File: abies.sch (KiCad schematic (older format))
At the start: 33 parts

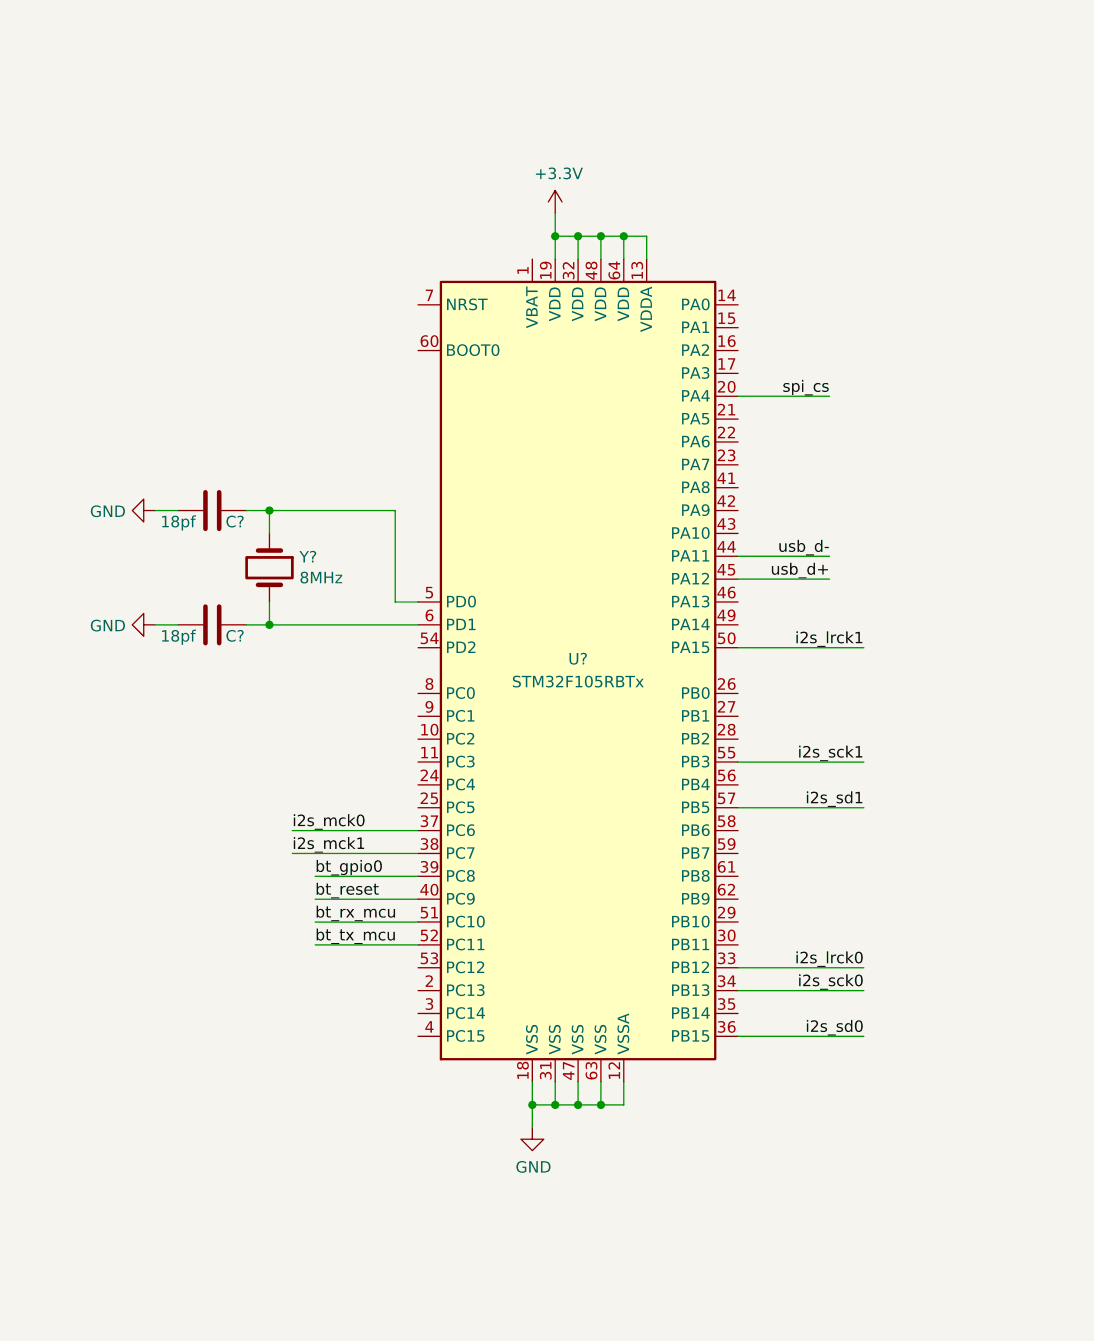
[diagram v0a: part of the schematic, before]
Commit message: Fix stuff. add psoc to sch
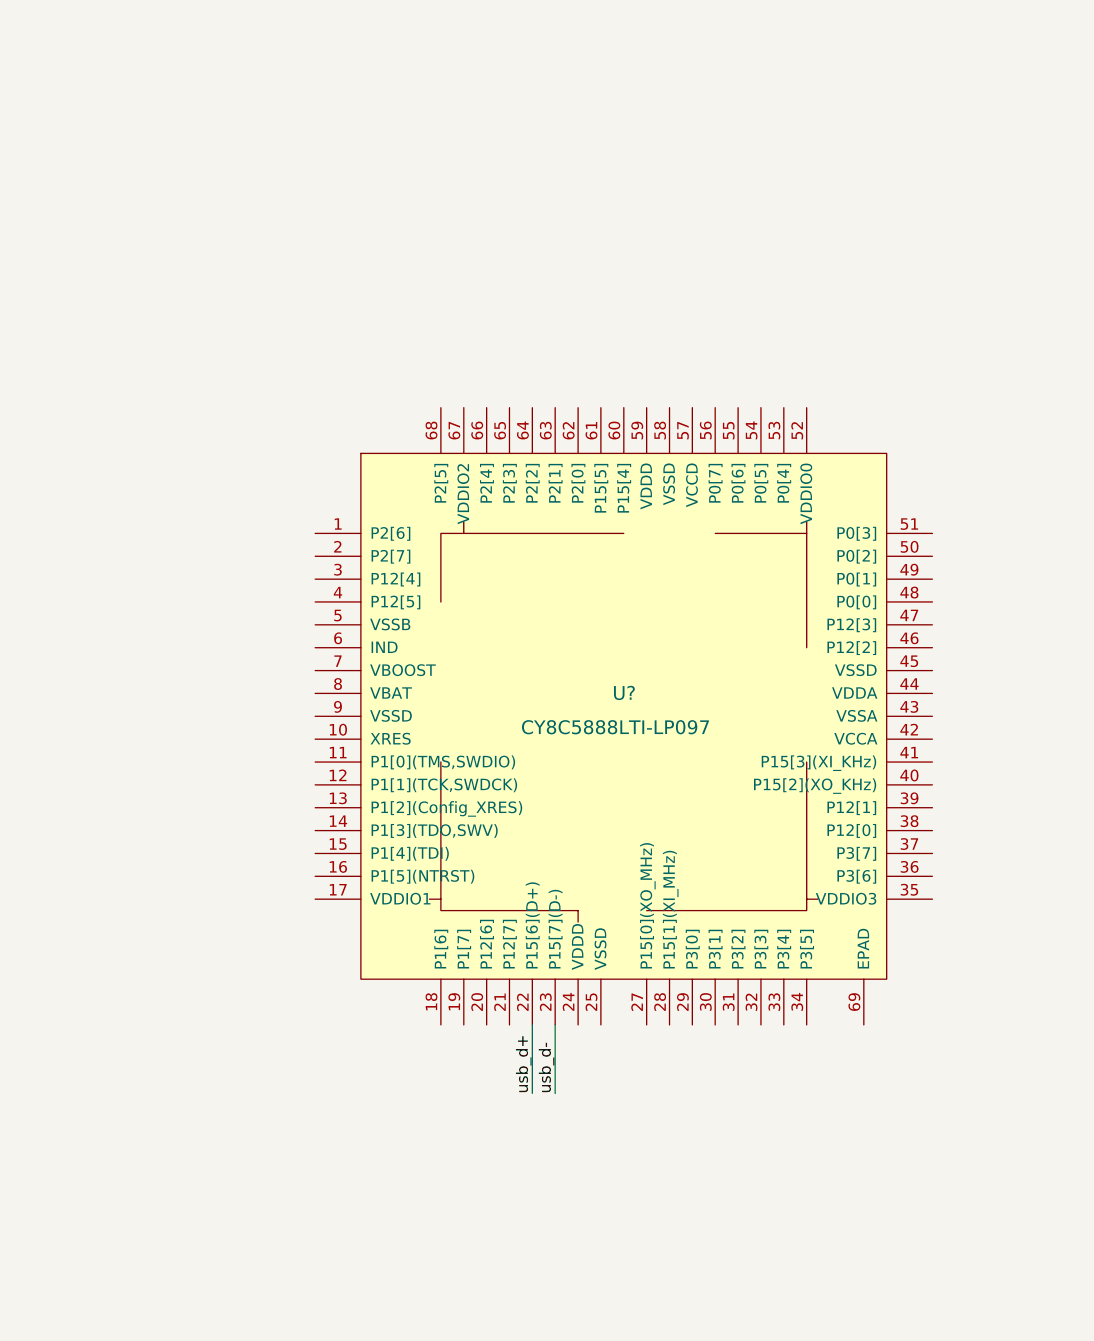
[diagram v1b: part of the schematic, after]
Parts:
- removed C? (x2): 18pf, symbol Device:C
- removed U?: STM32F105RBTx, Package_QFP:LQFP-64_10x10mm_P0.5mm, symbol MCU_ST_STM32F1:STM32F105RBTx
- removed Y?: 8MHz, symbol Device:Crystal
- added U?: CY8C5888LTI-LP097, Package_DFN_QFN:QFN-68-1EP_8x8mm_P0.4mm_EP5.2x5.2mm_ThermalVias, symbol microcontroller_arm:CY8C5888LTI-LP097
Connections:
- net usb_d+: now also U?.22 (P15[6](D+))
- net usb_d-: now also U?.23 (P15[7](D-))
- new net: U?.26 (VCCD), U?.57 (VCCD)
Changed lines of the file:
@@
 NoConn ~ 1300 2200
-$Comp
-L MCU_ST_STM32F1:STM32F105RBTx U?
-U 1 1 5ED74E5F
-P 3250 5650
-AR Path="/5ED36906/5ED74E5F" Ref="U?"  Part="1"
-AR Path="/5ED74E5F" Ref="U?"  Part="1"
-F 0 "U?" H 3250 5700 50  0000 C CNN
-F 1 "STM32F105RBTx" H 3250 5600 50  0000 C CNN
-F 2 "Package_QFP:LQFP-64_10x10mm_P0.5mm" H 2650 3950 50  0001 R CNN
-F 3 "http://www.st.com/st-web-ui/static/active/en/resource/technical/document/datasheet/CD00220364.pdf" H 3250 5650 50  0001 C CNN
-	1    3250 5650
-	1    0    0    -1
-$EndComp
-Text Label 4350 5250 2    50   ~ 0
-usb_d+
-Wire Wire Line
-	4350 5250 3950 5250
-Text Label 4350 5150 2    50   ~ 0
-usb_d-
-Wire Wire Line
-	4350 5150 3950 5150
-Text Label 2000 6350 0    50   ~ 0
-i2s_mck0
-Text Label 4500 7250 2    50   ~ 0
-i2s_sd0
-Text Label 4500 7050 2    50   ~ 0
-i2s_sck0
-Text Label 4500 6950 2    50   ~ 0
-i2s_lrck0
-Wire Wire Line
-	4500 6950 3950 6950
-Wire Wire Line
-	3950 7050 4500 7050
-Wire Wire Line
-	4500 7250 3950 7250
-Wire Wire Line
-	2000 6350 2550 6350
-Text Label 2000 6450 0    50   ~ 0
-i2s_mck1
-Wire Wire Line
-	2000 6450 2550 6450
-Text Label 4500 6050 2    50   ~ 0
-i2s_sck1
-Wire Wire Line
-	4500 6050 3950 6050
-Text Label 4500 5550 2    50   ~ 0
-i2s_lrck1
-Wire Wire Line
-	4500 5550 3950 5550
-Text Label 4500 6250 2    50   ~ 0
-i2s_sd1
-Wire Wire Line
-	4500 6250 3950 6250
-$Comp
-L Device:Crystal Y?
-U 1 1 5ED74E79
-P 1900 5200
-AR Path="/5ED36906/5ED74E79" Ref="Y?"  Part="1"
-AR Path="/5ED74E79" Ref="Y?"  Part="1"
-F 0 "Y?" V 1854 5331 50  0000 L CNN
-F 1 "8MHz" V 1945 5331 50  0000 L CNN
-F 2 "" H 1900 5200 50  0001 C CNN
-F 3 "~" H 1900 5200 50  0001 C CNN
-	1    1900 5200
-	0    1    1    0
-$EndComp
-Wire Wire Line
-	1900 5350 1900 5450
-Wire Wire Line
-	1900 5450 2550 5450
-Wire Wire Line
-	2550 5350 2450 5350
-Wire Wire Line
-	2450 5350 2450 4950
-Wire Wire Line
-	2450 4950 1900 4950
-Wire Wire Line
-	1900 4950 1900 5050
-$Comp
-L Device:C C?
-U 1 1 5ED74E85
-P 1650 5450
-AR Path="/5ED36906/5ED74E85" Ref="C?"  Part="1"
-AR Path="/5ED74E85" Ref="C?"  Part="1"
-F 0 "C?" V 1700 5550 50  0000 C CNN
-F 1 "18pf" V 1700 5300 50  0000 C CNN
-F 2 "" H 1688 5300 50  0001 C CNN
-F 3 "~" H 1650 5450 50  0001 C CNN
-	1    1650 5450
-	0    1    1    0
-$EndComp
-$Comp
-L Device:C C?
-U 1 1 5ED74E8B
-P 1650 4950
-AR Path="/5ED36906/5ED74E8B" Ref="C?"  Part="1"
-AR Path="/5ED74E8B" Ref="C?"  Part="1"
-F 0 "C?" V 1700 5050 50  0000 C CNN
-F 1 "18pf" V 1700 4800 50  0000 C CNN
-F 2 "" H 1688 4800 50  0001 C CNN
-F 3 "~" H 1650 4950 50  0001 C CNN
-	1    1650 4950
-	0    1    1    0
-$EndComp
-Wire Wire Line
-	1800 4950 1900 4950
-Connection ~ 1900 4950
-Wire Wire Line
-	1900 5450 1800 5450
-Connection ~ 1900 5450
-$Comp
-L power:GND #PWR?
-U 1 1 5ED74E95
-P 1400 5450
-AR Path="/5ED36906/5ED74E95" Ref="#PWR?"  Part="1"
-AR Path="/5ED74E95" Ref="#PWR?"  Part="1"
-F 0 "#PWR?" H 1400 5200 50  0001 C CNN
-F 1 "GND" V 1405 5322 50  0000 R CNN
-F 2 "" H 1400 5450 50  0001 C CNN
-F 3 "" H 1400 5450 50  0001 C CNN
-	1    1400 5450
-	0    1    1    0
-$EndComp
-Wire Wire Line
-	1400 5450 1500 5450
-$Comp
-L power:GND #PWR?
-U 1 1 5ED74E9C
-P 1400 4950
-AR Path="/5ED36906/5ED74E9C" Ref="#PWR?"  Part="1"
-AR Path="/5ED74E9C" Ref="#PWR?"  Part="1"
-F 0 "#PWR?" H 1400 4700 50  0001 C CNN
-F 1 "GND" V 1405 4822 50  0000 R CNN
-F 2 "" H 1400 4950 50  0001 C CNN
-F 3 "" H 1400 4950 50  0001 C CNN
-	1    1400 4950
-	0    1    1    0
-$EndComp
-Wire Wire Line
-	1400 4950 1500 4950
 $Comp
 L Device:R R?
@@
 	2700 1600 2600 1600
 Connection ~ 2600 1600
-$Comp
-L power:+3.3V #PWR?
-U 1 1 5ED976DD
-P 3150 3650
-F 0 "#PWR?" H 3150 3500 50  0001 C CNN
-F 1 "+3.3V" H 3165 3823 50  0000 C CNN
-F 2 "" H 3150 3650 50  0001 C CNN
-F 3 "" H 3150 3650 50  0001 C CNN
-	1    3150 3650
-	1    0    0    -1
-$EndComp
-Wire Wire Line
-	3150 3650 3150 3750
-Wire Wire Line
-	3150 3750 3250 3750
-Wire Wire Line
-	3450 3750 3450 3850
-Connection ~ 3150 3750
-Wire Wire Line
-	3150 3750 3150 3850
-Wire Wire Line
-	3350 3750 3350 3850
-Connection ~ 3350 3750
-Wire Wire Line
-	3350 3750 3450 3750
-Wire Wire Line
-	3250 3850 3250 3750
-Connection ~ 3250 3750
-Wire Wire Line
-	3250 3750 3350 3750
-Wire Wire Line
-	3450 3750 3550 3750
-Wire Wire Line
-	3550 3750 3550 3850
-Connection ~ 3450 3750
 Wire Notes Line
 	800  650  3050 650
@@
 Text Notes 800  650  0    50   ~ 0
 USB
-$Comp
-L power:GND #PWR?
-U 1 1 5EDA9575
-P 3050 7650
-AR Path="/5ED36906/5EDA9575" Ref="#PWR?"  Part="1"
-AR Path="/5EDA9575" Ref="#PWR?"  Part="1"
-F 0 "#PWR?" H 3050 7400 50  0001 C CNN
-F 1 "GND" H 3055 7477 50  0000 C CNN
-F 2 "" H 3050 7650 50  0001 C CNN
-F 3 "" H 3050 7650 50  0001 C CNN
-	1    3050 7650
-	1    0    0    -1
-$EndComp
-Wire Wire Line
-	3050 7450 3050 7550
-Wire Wire Line
-	3050 7550 3150 7550
-Wire Wire Line
-	3150 7550 3150 7450
-Connection ~ 3050 7550
-Wire Wire Line
-	3050 7550 3050 7650
-Wire Wire Line
-	3150 7550 3250 7550
-Wire Wire Line
-	3250 7550 3250 7450
-Connection ~ 3150 7550
-Wire Wire Line
-	3250 7550 3350 7550
-Wire Wire Line
-	3350 7550 3350 7450
-Connection ~ 3250 7550
-Wire Wire Line
-	3350 7550 3450 7550
-Wire Wire Line
-	3450 7550 3450 7450
-Connection ~ 3350 7550
 $Comp
 L audio_digital:CS4344 U?
@@
 Text Label 4150 1300 0    50   ~ 0
 bt_tx
-Text Label 2100 6750 0    50   ~ 0
-bt_rx_mcu
-Wire Wire Line
-	2100 6750 2550 6750
-Text Label 2100 6850 0    50   ~ 0
-bt_tx_mcu
-Wire Wire Line
-	2100 6850 2550 6850
 NoConn ~ 4650 1500
 NoConn ~ 4650 1600
@@
 NoConn ~ 5650 1400
 NoConn ~ 5650 1300
-Text Label 2100 6550 0    50   ~ 0
-bt_gpio0
-Wire Wire Line
-	2100 6550 2550 6550
-Text Label 2100 6650 0    50   ~ 0
-bt_reset
-Wire Wire Line
-	2100 6650 2550 6650
-Text Label 4350 4450 2    50   ~ 0
-spi_cs
-Wire Wire Line
-	4350 4450 3950 4450
 $Comp
 L Jumper:Jumper_3_Open JP?
@@
 Text Notes 9750 7000 0    50   ~ 0
 ADC
+$Comp
+L microcontroller_arm:CY8C5888LTI-LP097 U?
+U 1 1 5F1FE5BA
+P 3450 5850
+F 0 "U?" H 3400 5950 60  0000 L CNN
+F 1 "CY8C5888LTI-LP097" H 3000 5800 60  0000 L CNN
+F 2 "Package_DFN_QFN:QFN-68-1EP_8x8mm_P0.4mm_EP5.2x5.2mm_ThermalVias" H 2500 6650 60  0001 C CNN
+F 3 "https://www.cypress.com/file/45906/download" H 2500 6650 60  0001 C CNN
+F 4 "Cypress Semicondutor" H 5450 6050 60  0001 C CNN "Manufacturer"
+F 5 "CY8C5888LTI-LP097" H 5450 5950 60  0001 C CNN "Manufacturer Part Number"
+	1    3450 5850
+	1    0    0    -1
+$EndComp
+Text Label 3050 7500 1    50   ~ 0
+usb_d+
+Text Label 3150 7500 1    50   ~ 0
+usb_d-
+Wire Wire Line
+	3150 7500 3150 7200
+Wire Wire Line
+	3050 7200 3050 7500
 $EndSCHEMATC

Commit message: starting over.
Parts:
- removed C? (x2): 10uF, symbol Device:C
- removed C? (x2): 3.3uF, symbol Device:CP
- removed C? (x2): 10uF, symbol Device:CP
- removed C? (x2): 0.1uF, symbol Device:C
- removed C?: 1uF, symbol Device:CP
- removed F?: ~, symbol Device:Fuse
- removed FB?: ~, symbol Device:Ferrite_Bead
- removed J?: USB_B_Mini, symbol Connector:USB_B_Mini
- removed JP? (x2): Jumper_3_Open, symbol Jumper:Jumper_3_Open
- removed R? (x2): 22, symbol Device:R
- removed R? (x2): 10k, symbol Device:R
- removed R? (x2): 470, symbol Device:R
- removed U?: CS5340, Package_SO:TSSOP-16_4.4x5mm_P0.65mm, symbol audio_digital:CS5340
- removed U?: CMOD_A7, symbol fpga_dev:CMOD_A7
- removed U?: CS4344, Package_SO:TSSOP-10_3x3mm_P0.5mm, symbol audio_digital:CS4344
- removed U?: BGX13P, symbol bluetooth:BGX13P
- removed U?: CY8C5888LTI-LP097, Package_DFN_QFN:QFN-68-1EP_8x8mm_P0.4mm_EP5.2x5.2mm_ThermalVias, symbol microcontroller_arm:CY8C5888LTI-LP097
- added U?: CS5340, Package_SO:TSSOP-16_4.4x5mm_P0.65mm, symbol audio_digital:CS5340
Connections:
- net +3.3VA: now also U?.13 (VA)
- net +3V3: now also U?.3 (VL), U?.6 (VD)
- net GND: now also U?.14 (GND), U?.5 (GND)
- net adc_m0: now also U?.1 (M0)
- net adc_m1: now also U?.16 (M1)
- net adc_~rst~: now also U?.9 (~RST)
- net i2s_clk3: now also U?.2 (MCLK)
- net i2s_lrck3: now also U?.8 (LRCK)
- net i2s_sck3: now also U?.7 (SCLK)
- net i2s_sd3: now also U?.4 (SDOUT)
- net at C?.1, C?.2: now also U?.11 (VQ)
- net at C?.1, C?.2: now also U?.15 (FILT+)
- no-connect marks 8 -> 0
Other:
- note removed: "Bluetooth Comm"
- note removed: "Output Amplifier"
- note removed: "Stereo DAC"
- note removed: "USB"
- note removed: "i2s0: USB to FPGA Bridge\ni2s1: FPGA to USB Bridge\ni2s2: FPGA to DAC\ni2s3: ADC to FPGA"
- moved on the sheet: C?, R?
